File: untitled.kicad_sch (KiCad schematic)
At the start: 62 parts, among them IC5 HX711, IC6 HX711, IC7 HX711, IC8 HX711, J10 Conn_01x04, J15 Conn_01x04, J16 Conn_01x04, J2 Conn_01x04, J6 Conn_01x02, J7 Conn_01x02, Q2 MMBT4403, Q3 MMBT4403, Q4 MMBT4403, Q5 MMBT4403

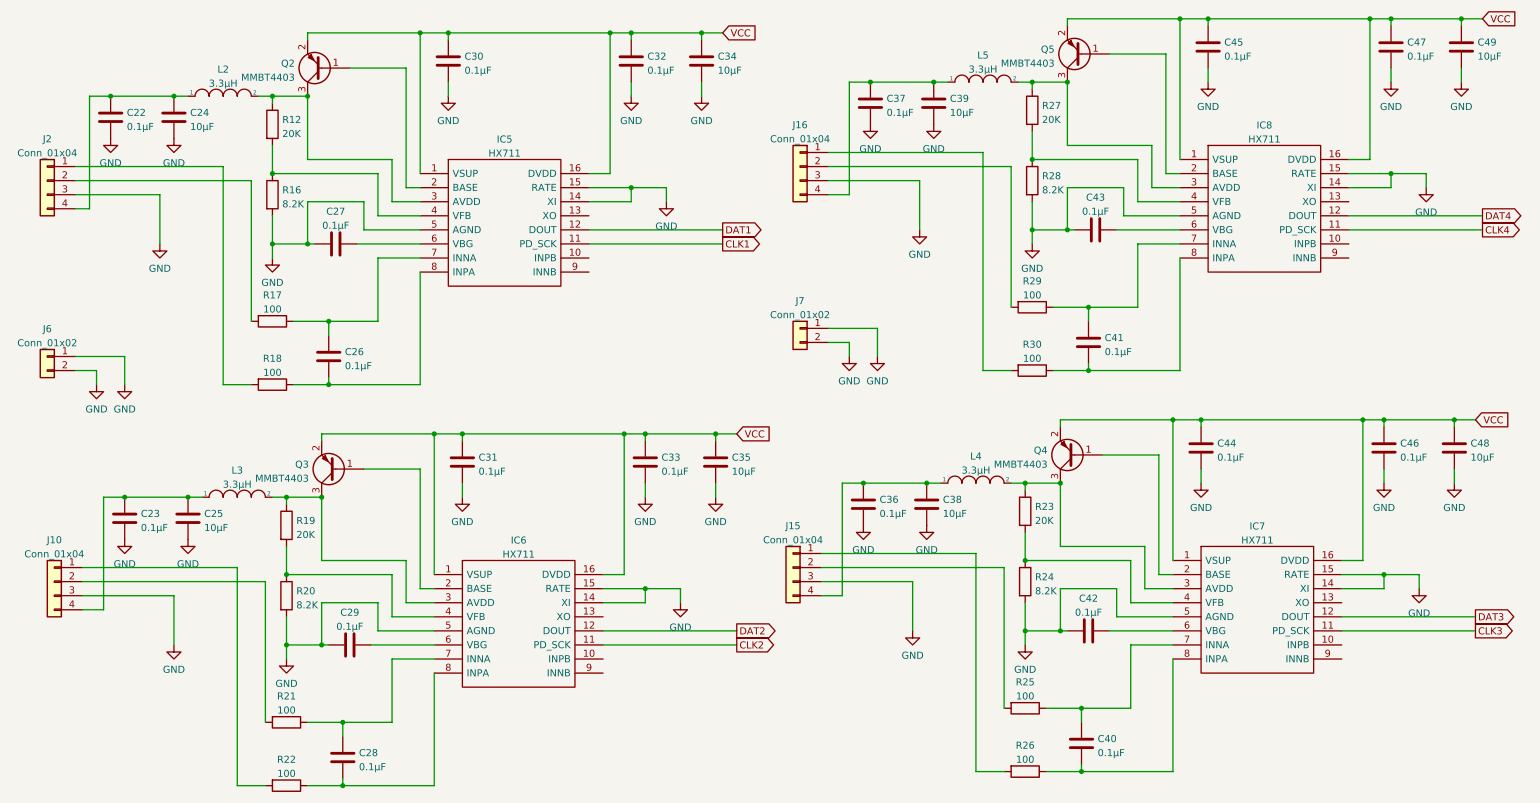
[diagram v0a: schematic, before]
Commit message: update
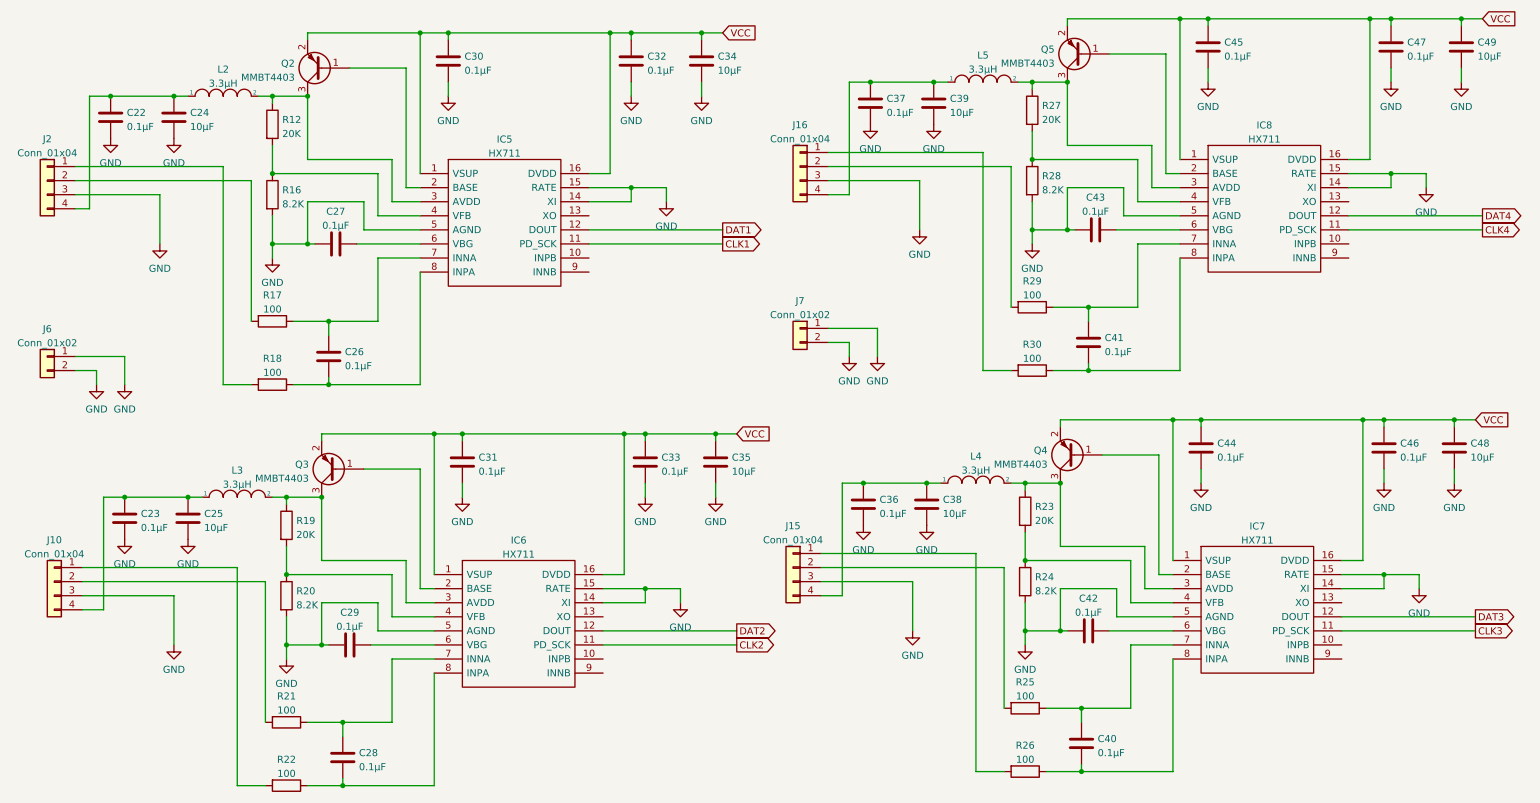
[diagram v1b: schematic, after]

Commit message: Revert "update"
This reverts commit 9afc669c055c7e8087787cb6fdf10dddd7845243.
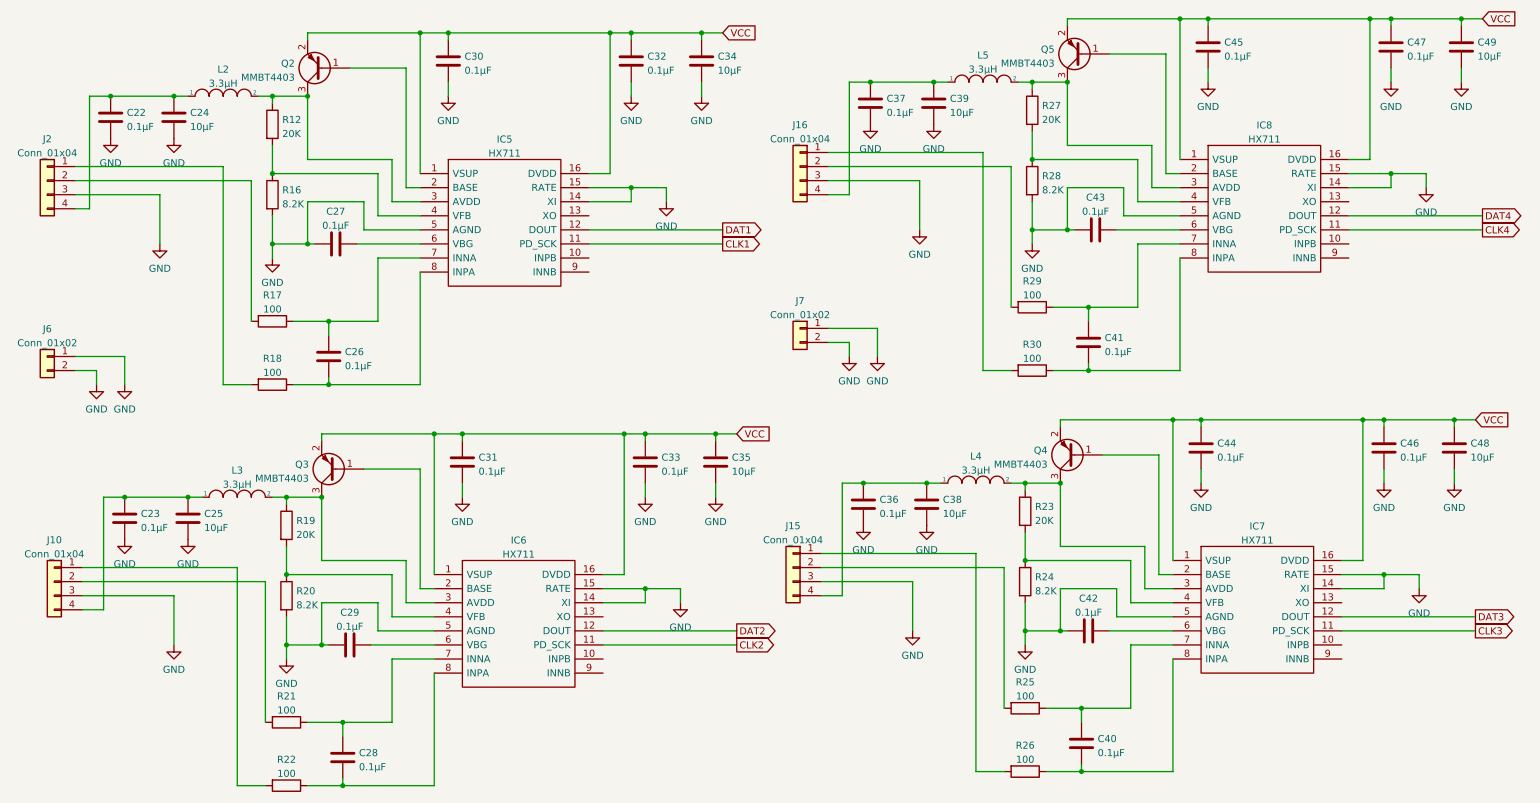
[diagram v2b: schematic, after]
